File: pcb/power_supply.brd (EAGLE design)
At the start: 39.4 x 68.4 mm, 40 parts, among them P1 2k, Q1 DIODES_FMMT493ATADIODES_FMMT4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, Q2 DIODES_FMMT493ATADIODES_FMMT4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, Q3 DIODES_FMMT493ATADIODES_FMMT4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, Q4 DIODES_FMMT493ATADIODES_FMMT4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, Q5 DIODES_FMMT493ATADIODES_FMMT4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, Q6 DIODES_FMMT493ATADIODES_FMMT4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, Q7 DIODES_FMMT493ATADIODES_FMMT4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, Q8 DIODES_FMMT493ATADIODES_FMMT4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, U1 LM1085IT-ADJ, U2 LM1085IT-ADJ

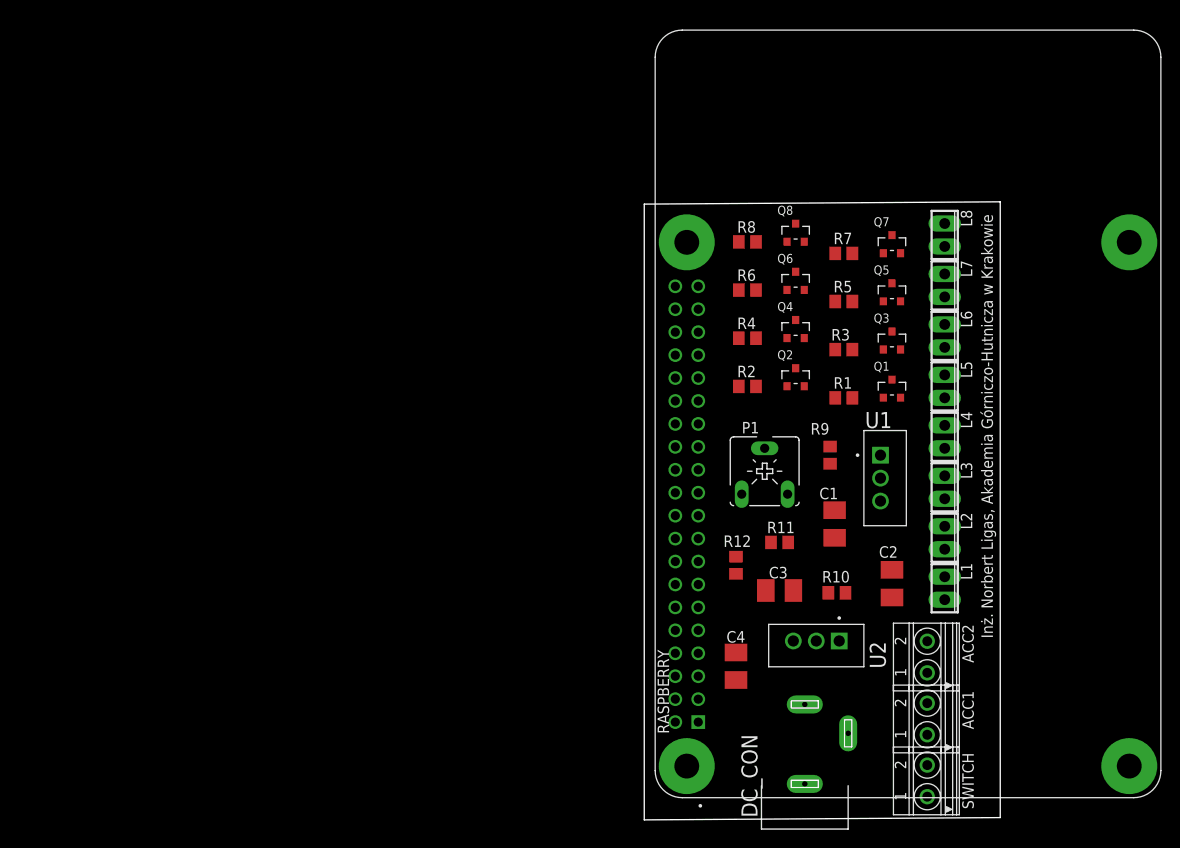
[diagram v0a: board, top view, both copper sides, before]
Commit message: pcb - board partially updated
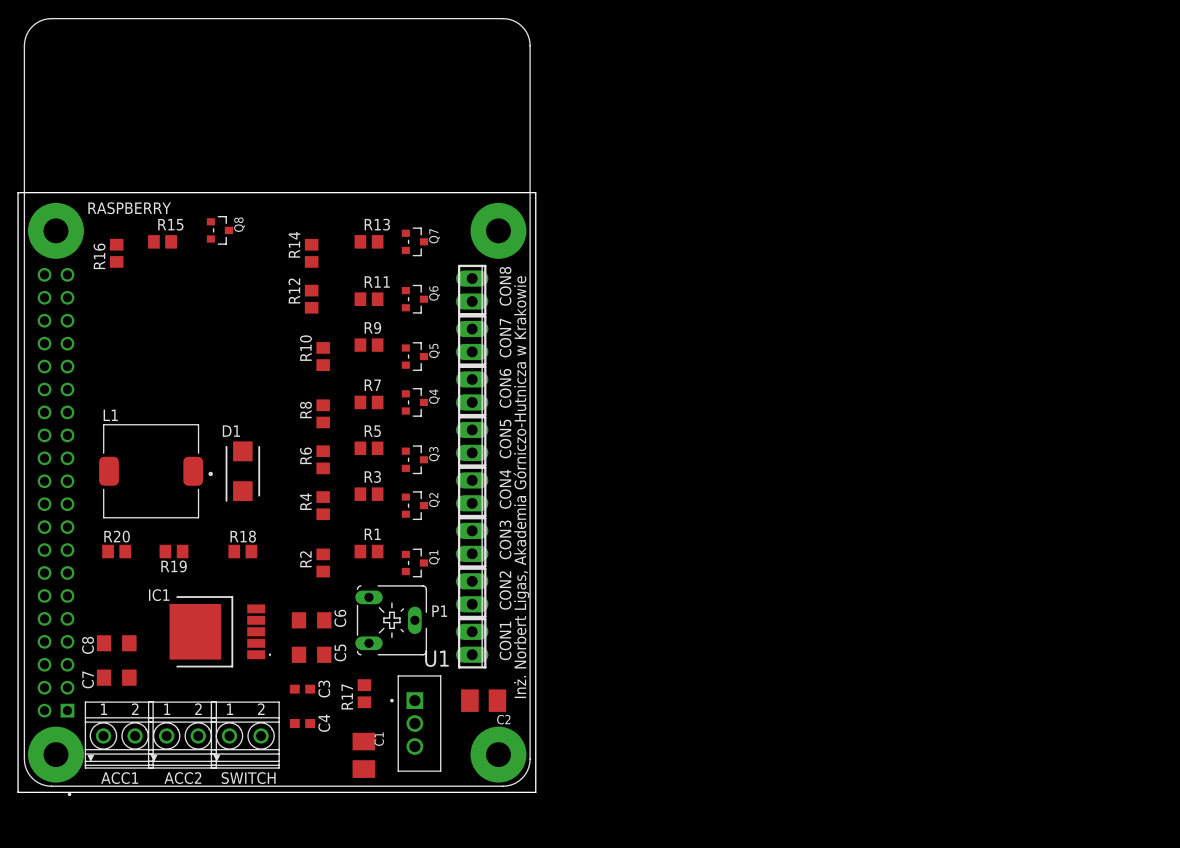
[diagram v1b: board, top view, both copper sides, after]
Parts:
- removed DC_CON: FC681478WURTH_694106301002, FC681478:WURTH_694106301002
- removed L2, L3, L4, L5, L6, L7, L8: (no value), con-phoenix-254:2POL254
- removed U2: LM1085IT-ADJ, LM1085IT-ADJ:TO254P1054X470X1955-3
- added C5, C6: 4.7u, rcl:C1206
- added C7, C8: 22u, rcl:C1206
- added CON1, CON2, CON3, CON4, CON5, CON6, CON7, CON8: +, con-phoenix-254:2POL254
- added D1: SSB44-E3_52T, SSB44-E3_52T:DIOM5436X244N
- added IC1: AP1507-D5-13, AP1507-D5-13:AP1507D513
- added R13, R15, R20: 4.3k, rcl:R0805
- added R14, R16: 22k, rcl:R0805
- added R17: 120, rcl:R0805
- added R18: 2.4k, rcl:R0805
- added R19: 3.3k, rcl:R0805
- C3, C4: value 10u -> 100n; device rcl:B/3528-21R -> rcl:C0603
- L1: value 1 -> HPI1040-220; device con-phoenix-254:2POL254 -> SRR1050A-151Y:INDM102100X510N
- R1, R3, R5, R7: value 100 -> 4.3k
- R10: value 120 -> 22k
- R11: value 330 -> 4.3k
- R12: value 39 -> 22k
- R2, R4, R6, R8: value 100 -> 22k
- R9: value 120 -> 4.3k
- moved ACC1 89.4 mm to (11.7, 7.61), turned to 0 degrees
- moved L1 88.8 mm to (15.2, 36.8), turned to 180 degrees
- moved ACC2 82.8 mm to (18.7, 7.61), turned to 0 degrees
- moved SWITCH 75.6 mm to (25.7, 7.61), turned to 0 degrees
- moved RASPBERRY 69.9 mm to (29.2, 44.5)
- moved Q8 63.8 mm to (22.9, 63.5), turned to 270 degrees
- moved R10 62.6 mm to (34.3, 49.5), turned to 90 degrees
- moved U1 58.3 mm to (44.5, 8.89)
- moved C1 58.1 mm to (38.8, 5.37)
- moved Q1 56.2 mm to (44.5, 26.7), turned to 270 degrees
- moved R12 55.5 mm to (33.0, 55.9)
- moved R1 55.3 mm to (39.4, 27.9)
- moved R7 55.1 mm to (39.4, 44.5)
- moved R5 55.0 mm to (39.4, 39.4)
- moved R3 55.0 mm to (39.4, 34.3)
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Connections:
- removed net 5V: C4.+, R10.2, RASPBERRY.2, RASPBERRY.4, U2.2
- removed net N$11: Q5.1, R5.2
- removed net N$12: L5.1, Q5.3
- removed net N$15: Q7.1, R7.2
- removed net N$16: L7.1, Q7.3
- removed net N$3 (its old number): ACC2.2, DC_CON.P$3
- removed net N$30: R11.1, R12.2
- removed net N$31: ACC1.1, DC_CON.P$1, SWITCH.2
- removed net N$8: L3.1, Q3.3
- new net N$32: D1.1, IC1.2, L1.1
- new net N$33: Q6.1, R11.2
- new net N$34: CON6.1, Q6.3
- new net N$37: Q7.1, R13.2
- new net N$38: CON7.1, Q7.3
- new net N$4: IC1.4, R18.2, R19.2
- new net N$41: Q8.1, R15.2
- new net N$42: CON8.1, Q8.3
- new net RASP_SUPPLY: C7.1, C8.1, L1.2, R20.1, RASPBERRY.2, RASPBERRY.4
- net BAT: now also C3.1, C4.1, C5.1, C6.1, IC1.1, SWITCH.2; no longer C3.+, SWITCH.1, U2.3
- net GND: now also ACC1.1, C3.2, C4.2, C5.2, C6.2, C7.2, C8.2, D1.2, IC1.3, IC1.5, IC1.6, R10.1, R14.1, R16.1, R18.1, R2.1, R4.1, R6.1, R8.1; no longer C3.-, C4.-, DC_CON.P$2
- net LIGHTS+: now also CON1.2, CON2.2, CON3.2, CON4.2, CON5.2, CON6.2, CON7.2, CON8.2, R17.2; no longer L1.2, L2.2, L3.2, L4.2, L5.2, L6.2, L7.2, L8.2, R9.2
- net N$1: now also CON1.1; no longer L1.1
- net N$10: now also CON3.1, Q3.3; no longer L4.1, Q4.3
- net N$13: now also Q4.1, R7.2; no longer Q6.1, R6.2
- net N$14: now also CON4.1, Q4.3; no longer L6.1, Q6.3
- net N$17: now also Q5.1, R9.2; no longer Q8.1, R8.2
- net N$18: now also CON5.1, Q5.3; no longer L8.1, Q8.3
- net N$19: now also R2.2
- net N$2: now also R19.1, R20.2; no longer R10.1, R11.2, U2.1
- net N$20: now also R3.1, R4.2; no longer R2.1
- net N$21: now also R5.1, R6.2; no longer R3.1
- net N$23: now also R7.1, R8.2; no longer R4.1
- net N$24: now also R10.2, R9.1; no longer R5.1
- net N$25: now also R11.1, R12.2; no longer R6.1
- net N$26: now also R13.1, R14.2; no longer R7.1
- net N$27: now also R15.1, R16.2; no longer R8.1
- net N$29: now also R17.1; no longer R9.1
- net N$5: now also R3.2; no longer R2.2
- net N$6: now also CON2.1; no longer L2.1
- net N$7: now also ACC2.2, SWITCH.1; no longer Q3.1, R3.2
- net N$9: now also Q3.1, R5.2; no longer Q4.1, R4.2
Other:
- board size 39.4 x 68.4 mm -> 57.3 x 66.4 mm
- board text removed: "+"
